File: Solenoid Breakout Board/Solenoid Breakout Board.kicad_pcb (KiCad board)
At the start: 2 copper layers, 106 parts, among them J1 Solenoid In, Q1 STN851-A, Q10 STN851-A, Q11 STN851-A, Q12 STN851-A, Q13 STN851-A, Q14 STN851-A, Q15 STN851-A, Q16 STN851-A, Q17 STN851-A, Q18 STN851-A, Q19 STN851-A, Q2 STN851-A, Q20 STN851-A, Q3 STN851-A, Q4 STN851-A, Q5 STN851-A, Q6 STN851-A, Q7 STN851-A, Q8 STN851-A, Q9 STN851-A, U1 LTV-247, U2 LTV-247, U3 LTV-247, U4 LTV-247, U5 LTV-247

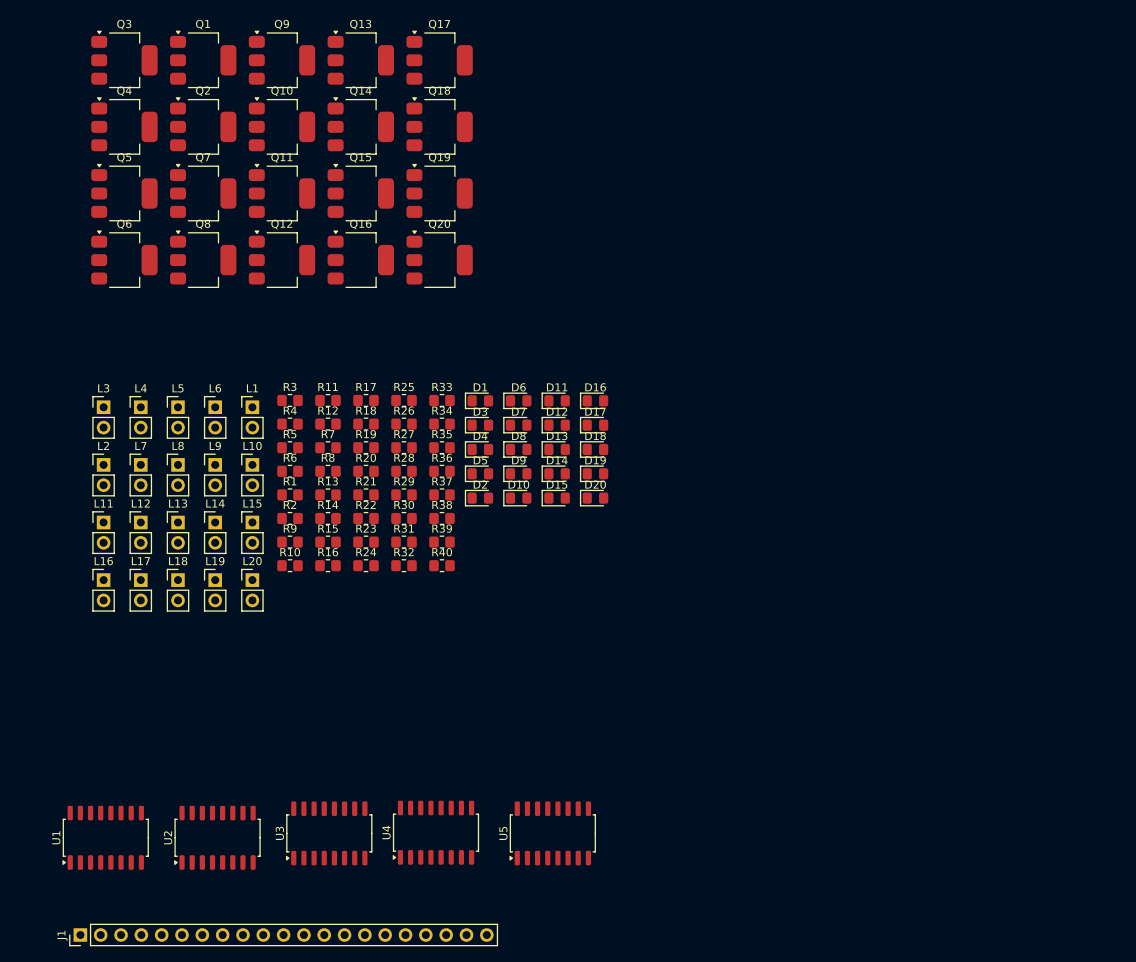
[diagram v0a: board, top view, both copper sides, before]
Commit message: finished rev A pcb for breakout:
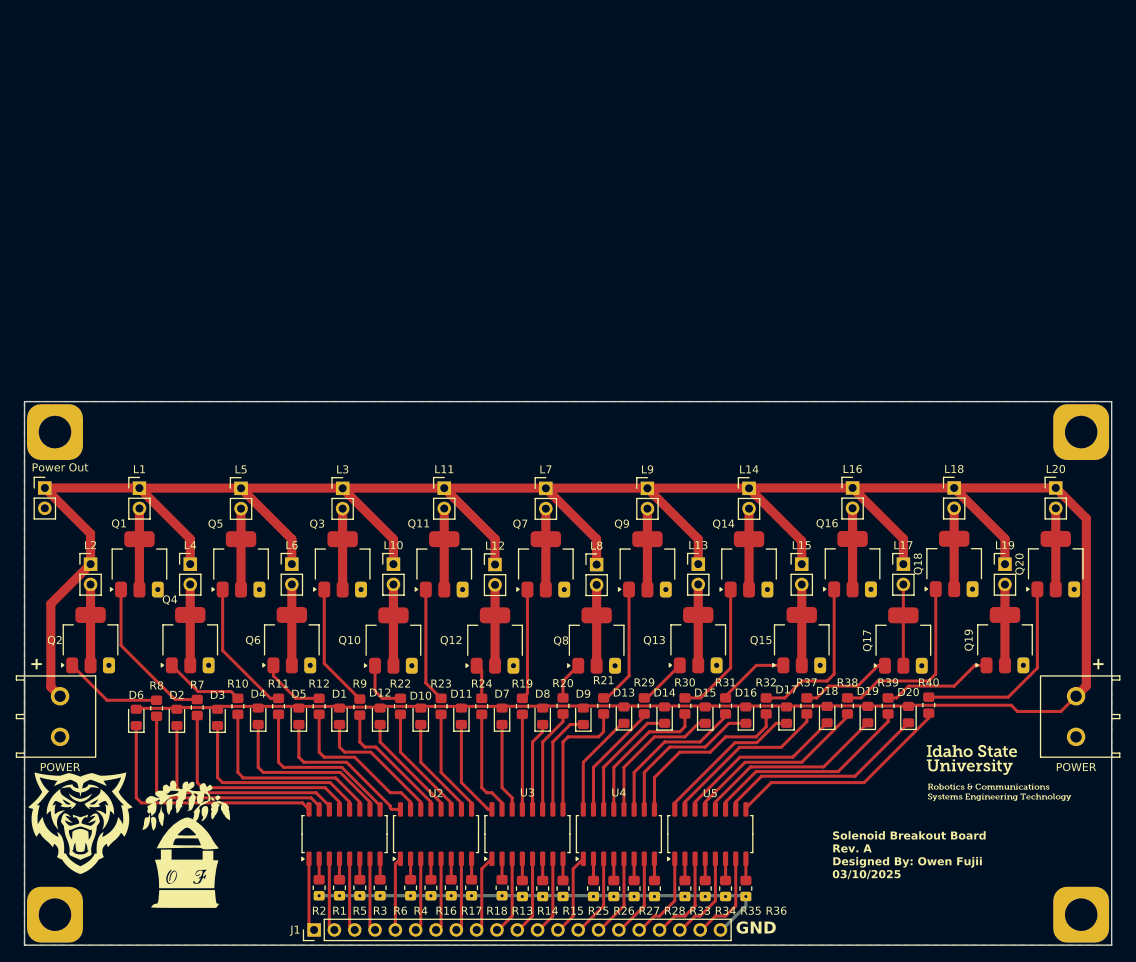
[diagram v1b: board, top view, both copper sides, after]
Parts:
- added G***: LOGO, Logos:ISU 1inch, F.Cu at (163.2, 134.0)
- added G***: LOGO, Logos:Bengal Head .5x.5, F.Cu at (51.4, 140.3)
- added G***: LOGO, Logos:Wisteria Logo .75x.75, F.Cu at (64.8, 142.9)
- added POWER: Two_Pin_Screw_Terminal, OF footprints:Two_Pin_Screw_Terminal, F.Cu at (175.9, 127.0)
- added POWER: Two_Pin_Screw_Terminal, OF footprints:Two_Pin_Screw_Terminal, F.Cu at (48.9, 127.0)
- added Power Out: Pwr IN, Connector_PinHeader_2.54mm:PinHeader_1x02_P2.54mm_Vertical, F.Cu at (47.0, 98.4)
- added REF**: 6-32 Mount, OF footprints:6-32 Mount, F.Cu at (176.5, 91.4)
- added REF**: 6-32 Mount, OF footprints:6-32 Mount, F.Cu at (48.3, 91.4)
- added REF**: 6-32 Mount, OF footprints:6-32 Mount, F.Cu at (176.5, 151.8)
- added REF**: 6-32 Mount, OF footprints:6-32 Mount, F.Cu at (48.3, 151.8)
- moved L20 101.1 mm to (173.4, 98.4)
- moved L19 98.7 mm to (167.0, 108.0)
- moved L18 97.7 mm to (160.7, 98.4)
- moved L17 95.3 mm to (154.3, 108.0)
- moved L16 94.3 mm to (148.0, 98.4)
- moved Q17 92.9 mm to (154.3, 117.5), turned to 90 degrees
- moved Q19 90.1 mm to (167.0, 117.5), turned to 90 degrees
- moved Q20 85.9 mm to (173.4, 108.0), turned to 90 degrees
- moved Q18 84.4 mm to (160.7, 107.9), turned to 90 degrees
- moved Q13 83.9 mm to (128.7, 117.5), turned to 90 degrees
- moved Q15 78.5 mm to (141.6, 117.5), turned to 90 degrees
- moved Q9 77.8 mm to (122.3, 108.0), turned to 90 degrees
- moved Q14 73.1 mm to (135.0, 108.0), turned to 90 degrees
- moved Q16 72.3 mm to (148.0, 108.0), turned to 90 degrees
- moved L15 68.9 mm to (141.6, 108.0)
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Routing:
- net +12v: track 0.00 -> 416.3 mm
- net GND: track 0.00 -> 59.0 mm
- net Net-(D6-K): track 0.00 -> 31.2 mm
- net Net-(R8-Pad1): track 0.00 -> 31.0 mm
- net Net-(R40-Pad1): track 0.00 -> 28.3 mm
- net Net-(D2-K): track 0.00 -> 28.2 mm
- net Net-(R7-Pad1): track 0.00 -> 28.1 mm
- net Net-(D20-K): track 0.00 -> 26.6 mm
- net Net-(R39-Pad1): track 0.00 -> 26.4 mm
- net Net-(D3-K): track 0.00 -> 25.2 mm
- net Net-(R10-Pad1): track 0.00 -> 25.0 mm
- net Net-(Q20-B): track 0.00 -> 24.9 mm
- net Net-(D19-K): track 0.00 -> 24.1 mm
- net Net-(R38-Pad1): track 0.00 -> 23.5 mm
- net Net-(Q18-B): track 0.00 -> 22.9 mm
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- added copper zone on B.Cu, net Chassis_GND
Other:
- board outline added: 135.9 x 67.9 mm
- board text added: "+"
- board text added: "GND"
- board text added: "Solenoid Breakout Board Rev. A Designed By: Owen Fujii 03/10/2025"
